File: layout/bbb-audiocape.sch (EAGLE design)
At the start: 39 parts, among them U1 TLV320AIC3104, U2 V_REG_LDOSMD

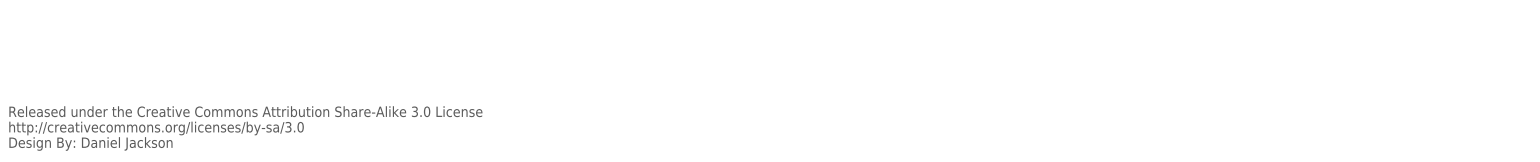
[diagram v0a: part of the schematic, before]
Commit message: Added docu pic, Added License stuff
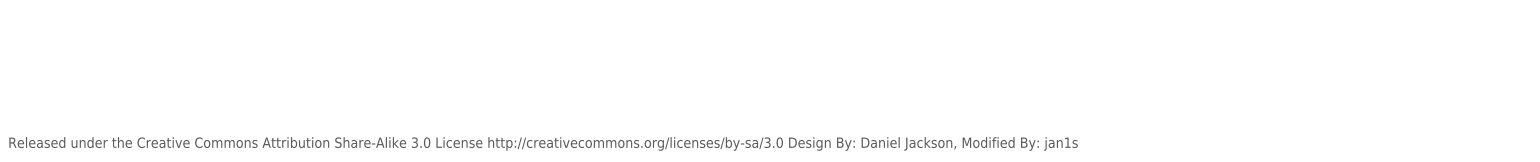
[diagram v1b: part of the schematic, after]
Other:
- note added: "Released under the Creative Commons Attribution Share-Alike 3.0 License http://creativecommons.org/licenses/by-sa/3.0 Design By: Daniel Jackson, Modified By: jan1s"
- note removed: "Released under the Creative Commons Attribution Share-Alike 3.0 License http://creativecommons.org/licenses/by-sa/3.0 Design By: Daniel Jackson"
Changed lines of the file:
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@@
 <sheet>
 <plain>
-<text x="-149.86" y="-58.42" size="2.54" layer="97">Released under the Creative Commons Attribution Share-Alike 3.0 License
-http://creativecommons.org/licenses/by-sa/3.0
-Design By: Daniel Jackson</text>
+<text x="-149.86" y="-58.42" size="2.54" layer="97">Released under the Creative Commons Attribution Share-Alike 3.0 License http://creativecommons.org/licenses/by-sa/3.0 Design By: Daniel Jackson, Modified By: jan1s</text>
 </plain>
 <instances>
